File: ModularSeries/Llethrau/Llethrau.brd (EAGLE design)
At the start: 48.5 x 100 mm, 20 parts, among them SW1 SPDT_SWITCHDW1

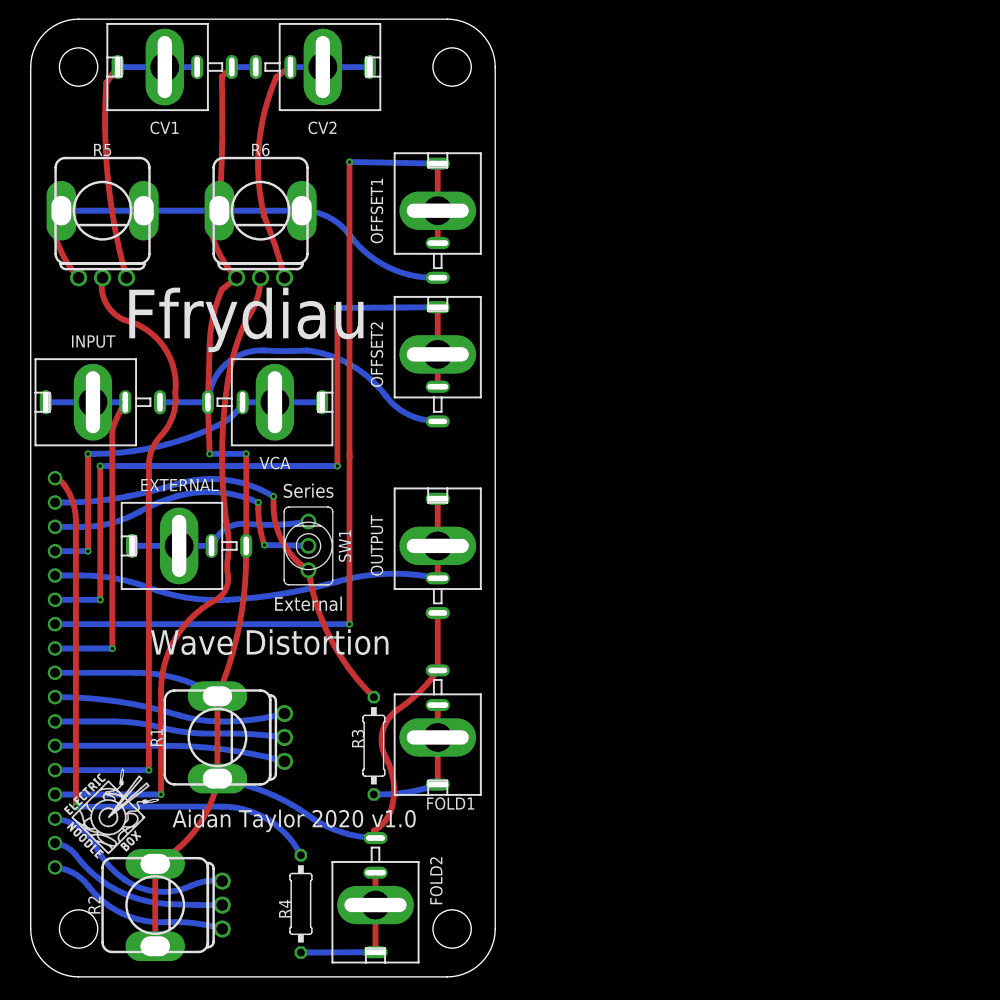
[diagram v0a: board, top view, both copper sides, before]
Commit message: Fields added and various updates to designs
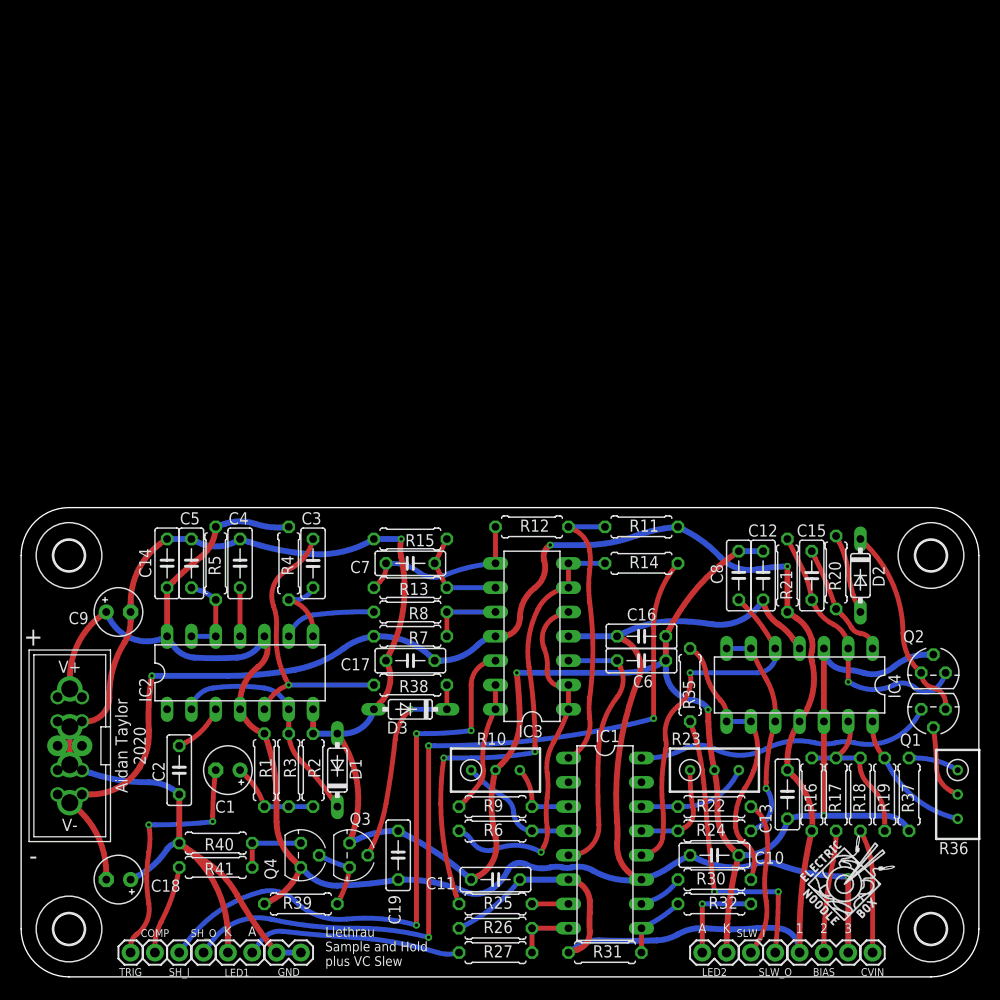
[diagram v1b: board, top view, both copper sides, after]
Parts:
- removed BOARD1: FFRYDIAU_LINK, ElectricNoodleBox:FFRYDIAU
- removed CV1, CV2, EXTERNAL, FOLD1, FOLD2, INPUT, OFFSET1, OFFSET2, OUTPUT, VCA: COMBI-JACKCINCHNANA, ElectricNoodleBox:NEWCOMBOJACK_PANEL
- removed SW1: SPDT_SWITCHDW1, ElectricNoodleBox:MICRODPDT-DW1
- added BIAS: 3XWIREPAD, ElectricNoodleBox:1X03
- added C1: 4.7µF, rcl:E2,5-5
- added C10, C11, C12, C13, C14, C16, C17, C19, C5: 100nF, rcl:C050-025X075
- added C15: 10pF, rcl:C050-025X075
- added C18, C9: 10µF, rcl:E2,5-5
- added C2, C4, C8: 10nF, rcl:C050-025X075
- added C3: 2.2nF, rcl:C050-025X075
- added C6: 10nF PET, rcl:C050-025X075
- added C7: 22pF, rcl:C050-025X075
- added COMP, CVIN, SH_I, SH_O, SLW_I, SLW_O, TRIG: 1XWIREPAD, ElectricNoodleBox:1X01
- added D1, D2, D3: BAT85, ElectricNoodleBox:DO35-7
- added GND, LED1, LED2: 2XWIREPAD, ElectricNoodleBox:1X02
- added H1, H2, H3, H4: MOUNT-HOLE3.2, holes:3,2
- added IC1: (no value), ElectricNoodleBox:DIL16
- added IC2: 556_DUALTIMERDIL14, ElectricNoodleBox:DIL14
- added IC3, IC4: (no value), ElectricNoodleBox:DIL14
- added Q1, Q2: 2N3906, transistor-pnp:TO92
- added Q3, Q4: 2N3904, transistor-npn:TO92
- added R10, R23, R36: 10K, rcl:RTRIM3296W
- added R11: 4K7, rcl:0207/7
- added R12, R22, R24, R9: 10K, rcl:0207/7
- added R13, R15, R16, R17, R18, R25, R30, R7, R8: 100K, rcl:0207/7
- added R14, R26, R31, R35, R41: 1K, rcl:0207/7
- added R19, R27, R32: 2K, rcl:0207/7
- added R20: 47K, rcl:0207/7
- added R21: 1M, rcl:0207/7
- added R37: 75Ω, rcl:0207/7
- added R38, R39: 15K, rcl:0207/7
- added R40: 470Ω, rcl:0207/7
- added WP1: COMBO_SUPPLY_HEADER, ElectricNoodleBox:COMBINED_POWER
- R1, R2: value B100K -> 100K; device ElectricNoodleBox:ALPHA_RV09_9MMPOT -> rcl:0207/7
- R3: value 100Ω -> 10K; device rcl:0207/10 -> rcl:0207/7
- R4: value 100Ω -> 20K; device rcl:0207/10 -> rcl:0207/7
- R5: value B100K -> 1K; device ElectricNoodleBox:ALPHA_RV09_9MMPOT -> rcl:0207/7
- R6: value B100K -> 10K; device ElectricNoodleBox:ALPHA_RV09_9MMPOT -> rcl:0207/7
- moved U$1 77.2 mm to (81.3, 5.08)
- moved R6 69.3 mm to (49.5, 15.2)
- moved U$2 58.6 mm to (90.8, 5.08)
- moved R5 38.7 mm to (20.3, 43.2), turned to 90 degrees
- moved R4 35.6 mm to (27.9, 43.2), turned to 90 degrees
- moved R2 21.7 mm to (30.5, 21.6), turned to 270 degrees
- moved R3 9.25 mm to (27.9, 21.6)
- moved R1 5.97 mm to (25.4, 21.6)
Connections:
- new net +12V: BIAS.3, C10.1, C12.1, C14.1, C16.1, C19.1, C9.+, IC1.11, IC2.10, IC2.14, IC2.4, IC3.4, IC4.4, Q4.1, R1.2, R39.1, R4.2, R5.2, WP1.V+1, WP1.V+2, WP1.V+3
- new net -12V: BIAS.1, C11.2, C13.2, C17.2, C18.-, IC1.6, IC3.11, IC4.11, R11.2, R16.2, R21.1, R26.2, R31.2, R7.2, WP1.V-1, WP1.V-2, WP1.V-3
- new net N$18: C1.-, TRIG.1
- new net N$23: C7.1, IC3.9, R13.2, R15.1
- new net N$24: IC4.13, R16.1, R17.1, R18.1, R19.2
- new net N$25: IC4.14, R19.1, R36.3
- new net N$26: D2.A, R20.2
- new net N$27: IC4.10, IC4.6, IC4.7, R24.2
- new net N$28: BIAS.2, R17.2
- new net N$29: CVIN.1, R18.2
- new net N$30: IC1.14, R22.2, R23.3
- new net N$31: R36.1, R37.1
- new net N$32: Q1.2, R36.2
- new net N$33: IC1.13, R23.1, R24.1
- new net N$34: COMP.1, R41.2
- new net N$35: D3.C, Q3.2, R38.2
- new net N$36: C8.1, IC1.12, IC4.5
- new net N$37: IC1.16, Q1.1
- new net N$38: IC4.8, IC4.9, R30.2, R35.1
- new net N$39: IC1.7, R25.1
- new net N$40: IC1.8, R26.1, R27.1
- new net N$41: LED2.1, R32.1
- new net N$42: IC1.10, R30.1
- new net N$43: IC1.9, R31.1, R32.2
- new net N$45: R35.2, SLW_O.1
- new net N$46: C15.1, IC4.1, R20.1
- new net N$47: C15.2, IC4.2, Q2.1, R21.2
- new net N$48: R22.1, SLW_I.1
- new net N$49: Q3.1, Q4.2, R39.2
- new net N$50: Q4.3, R40.1, R41.1
- net AGND: now also C10.2, C11.1, C12.2, C13.1, C14.2, C16.2, C17.1, C18.+, C19.2, C2.2, C4.2, C5.2, C6.2, C8.2, C9.-, D1.A, D3.A, GND.1, GND.2, IC2.7, IC4.12, IC4.3, LED1.2, LED2.2, Q2.2, Q3.3, R10.2, R15.2, R2.1, R23.2, R37.2, R40.2, WP1.GND1, WP1.GND2, WP1.GND3, WP1.GND4, WP1.GND5, WP1.GND6, WP1.GND7, WP1.GND8; no longer BOARD1.GND, CV1.S, CV2.S, EXTERNAL.S, FOLD1.S, FOLD2.S, INPUT.S, OFFSET1.S, OFFSET2.S, OUTPUT.S, R1.LUGL, R1.LUGR, R2.LUGL, R2.LUGR, R5.C1, R5.LUGL, R5.LUGR, R6.C1, R6.LUGL, R6.LUGR, VCA.S
- net N$1: now also D1.C, IC2.2, IC2.6, R3.1; no longer CV1.CONN, CV1.T1, CV1.T2, R5.C3
- net N$10: now also IC3.10, R7.1, R8.1; no longer BOARD1.POT1_3, R1.C3
- net N$11: now also C7.2, IC3.8, R12.1, R13.1; no longer BOARD1.POT2_2, R2.C2
- net N$12: now also C6.1, IC1.5, IC3.3; no longer BOARD1.POT2_3, R2.C3
- net N$13: now also IC3.1, IC3.2, IC3.5, R6.1; no longer BOARD1.POT2_1, R2.C1
- net N$14: now also IC1.1, R11.1, R12.2; no longer BOARD1.SWITCH_S, R3.1, SW1.C1
- net N$15: now also IC1.4, R10.1, R6.2; no longer FOLD1.CONN, FOLD1.T1, FOLD1.T2, R3.2
- net N$16: now also IC1.3, R10.3, R9.1; no longer BOARD1.SWITCH_R, SW1.C2
- net N$17: now also IC3.13, IC3.14, R9.2; no longer EXTERNAL.CONN, EXTERNAL.T1, EXTERNAL.T2, SW1.C3
- net N$19: now also IC3.12, SH_I.1; no longer BOARD1.FOLD2, R4.1
- net N$2: now also C1.+, R1.1, R2.2, R3.2; no longer BOARD1.CV1, R5.C2
- net N$20: now also IC3.6, IC3.7, R14.1, R25.2; no longer FOLD2.CONN, FOLD2.T1, FOLD2.T2, R4.2
- net N$21: now also R14.2, SH_O.1; no longer CV2.CONN, CV2.T1, CV2.T2, R6.C3
- net N$22: now also D2.C, Q1.3, Q2.3; no longer BOARD1.CV2, R6.C2
- net N$3: now also LED1.1, R27.2; no longer BOARD1.SIG, INPUT.CONN, INPUT.T1, INPUT.T2
- net N$4: now also C3.1, IC2.5, R38.1; no longer BOARD1.OUT, OUTPUT.CONN, OUTPUT.T1, OUTPUT.T2
- net N$5: now also C5.1, IC2.12, IC2.13, R5.1; no longer BOARD1.POT1_2, R1.C2
- net N$6: now also C2.1, IC2.3; no longer BOARD1.OFS1, OFFSET1.CONN, OFFSET1.T1, OFFSET1.T2
- net N$7: now also C3.2, IC2.8, R4.1; no longer BOARD1.OFS2, OFFSET2.CONN, OFFSET2.T1, OFFSET2.T2
- net N$8: now also C4.1, IC2.11; no longer BOARD1.VCA, VCA.CONN, VCA.T1, VCA.T2
- net N$9: now also IC2.9, R8.2; no longer BOARD1.POT1_1, R1.C1
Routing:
- net +12V: track 0.00 -> 206.3 mm, vias 0 -> 1
- net -12V: track 0.00 -> 194.8 mm, vias 0 -> 3
- net N$6: track 96.5 -> 5.43 mm, vias 2 -> 0
- net N$7: track 78.7 -> 7.63 mm, vias 4 -> 0
- net AGND: track 246.6 -> 313.3 mm, vias 2 -> 4
- net N$2: track 63.9 -> 9.68 mm, vias 1 -> 0
- net N$21: track 31.4 -> 85.0 mm, vias 0 -> 3
- net N$22: track 67.4 -> 20.1 mm, vias 1 -> 0
- net N$36: track 0.00 -> 37.2 mm, vias 0 -> 1
- net N$8: track 39.3 -> 5.08 mm, vias 2 -> 0
- net N$20: track 16.1 -> 50.3 mm, vias 0 -> 2
- net N$45: track 0.00 -> 31.0 mm, vias 0 -> 2
- net N$37: track 0.00 -> 30.2 mm
- net N$38: track 0.00 -> 28.5 mm
- net N$47: track 0.00 -> 27.9 mm, vias 0 -> 1
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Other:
- board size 48.5 x 100 mm -> 100 x 49 mm
- board text added: "+"
- board text added: "-"
- board text added: "1"
- board text added: "2"
- board text added: "3"
- board text added: "A"
- board text added: "Aidan Taylor 2020"
- board text added: "K"
- board text added: "Llethrau Sample and Hold plus VC Slew"
- board text removed: "Aidan Taylor 2020 v1.0"
- board text removed: "External"
- board text removed: "Ffrydiau"
- board text removed: "Series"
- board text removed: "Wave Distortion"
